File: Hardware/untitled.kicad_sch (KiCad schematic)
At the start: 7 parts, among them U8 BMP280

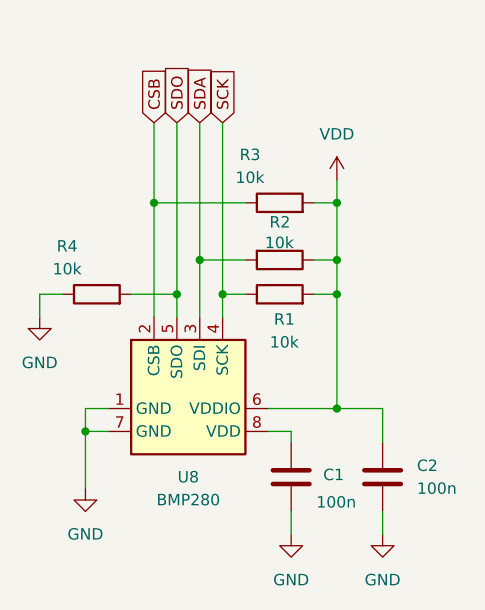
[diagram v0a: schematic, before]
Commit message: design sensores pronto
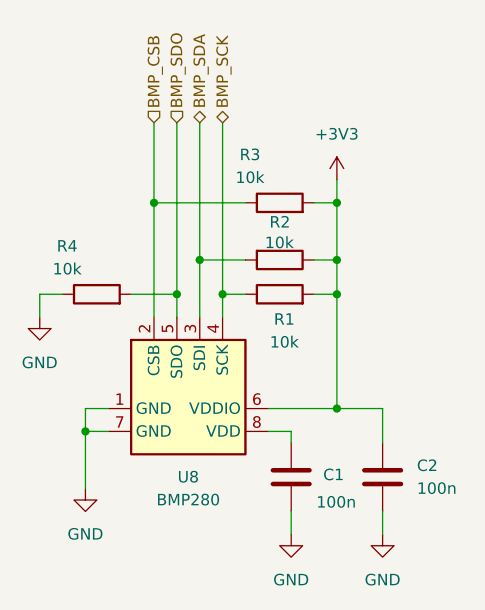
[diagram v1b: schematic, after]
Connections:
- net CSB renamed BMP_CSB
- net SCK renamed BMP_SCK
- net SDA renamed BMP_SDA
- net SDO renamed BMP_SDO
- net VDD renamed +3V3
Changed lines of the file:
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@@
 		)
 	)
-	(global_label "SDO"
+	(hierarchical_label "BMP_SDO"
 		(shape input)
 		(at 139.7 74.93 90)
-		(fields_autoplaced yes)
 		(effects
 			(font
@@
 			(justify left)
 		)
-		(property "Intersheetrefs" "${INTERSHEET_REFS}"
-			(at 139.7 68.1348 90)
-			(effects
-				(font
-					(size 1.27 1.27)
-				)
-				(justify left)
-				(hide yes)
-			)
-		)
-	)
-	(global_label "SDA"
-		(shape input)
+	)
+	(hierarchical_label "BMP_SDA"
+		(shape bidirectional)
 		(at 142.24 74.93 90)
-		(fields_autoplaced yes)
 		(effects
 			(font
@@
 			(justify left)
 		)
-		(property "Intersheetrefs" "${INTERSHEET_REFS}"
-			(at 142.24 68.3767 90)
-			(effects
-				(font
-					(size 1.27 1.27)
-				)
-				(justify left)
-				(hide yes)
-			)
-		)
-	)
-	(global_label "CSB"
+	)
+	(hierarchical_label "BMP_CSB"
 		(shape input)
 		(at 137.16 74.93 90)
-		(fields_autoplaced yes)
 		(effects
 			(font
@@
 			(justify left)
 		)
-		(property "Intersheetrefs" "${INTERSHEET_REFS}"
-			(at 137.16 68.1953 90)
-			(effects
-				(font
-					(size 1.27 1.27)
-				)
-				(justify left)
-				(hide yes)
-			)
-		)
-	)
-	(global_label "SCK"
-		(shape input)
+	)
+	(hierarchical_label "BMP_SCK"
+		(shape bidirectional)
 		(at 144.78 74.93 90)
-		(fields_autoplaced yes)
 		(effects
 			(font
@@
 			)
 			(justify left)
-		)
-		(property "Intersheetrefs" "${INTERSHEET_REFS}"
-			(at 144.78 68.1953 90)
-			(effects
-				(font
-					(size 1.27 1.27)
-				)
-				(justify left)
-				(hide yes)
-			)
 		)
 	)
@@
 	)
 	(symbol
+		(lib_id "power:+3V3")
+		(at 157.48 81.28 0)
+		(unit 1)
+		(exclude_from_sim no)
+		(in_bom yes)
+		(on_board yes)
+		(dnp no)
+		(fields_autoplaced yes)
+		(property "Reference" "#PWR015"
+			(at 157.48 85.09 0)
+			(effects
+				(font
+					(size 1.27 1.27)
+				)
+				(hide yes)
+			)
+		)
+		(property "Value" "+3V3"
+			(at 157.48 76.2 0)
+			(effects
+				(font
+					(size 1.27 1.27)
+				)
+			)
+		)
+		(property "Footprint" ""
+			(at 157.48 81.28 0)
+			(effects
+				(font
+					(size 1.27 1.27)
+				)
+				(hide yes)
+			)
+		)
+		(property "Datasheet" ""
+			(at 157.48 81.28 0)
+			(effects
+				(font
+					(size 1.27 1.27)
+				)
+				(hide yes)
+			)
+		)
+		(property "Description" "Power symbol creates a global label with name \"+3V3\""
+			(at 157.48 81.28 0)
+			(effects
+				(font
+					(size 1.27 1.27)
+				)
+				(hide yes)
+			)
+		)
+		(pin "1"
+		)
+		(instances
+			(project ""
+				(path "/0c305a6e-f9cd-49a1-b146-c2956e5469b6/0abc4084-0cd9-43a4-88f9-87e0e6566acc"
+					(reference "#PWR015")
+					(unit 1)
+				)
+			)
+		)
+	)
+	(symbol
 		(lib_id "Device:R")
 		(at 151.13 90.17 270)
@@
 					(unit 1)
 				)
-			)
-		)
-	)
-	(symbol
-		(lib_id "power:VDD")
-		(at 157.48 81.28 0)
-		(unit 1)
-		(exclude_from_sim no)
-		(in_bom yes)
-		(on_board yes)
-		(dnp no)
-		(fields_autoplaced yes)
-		(property "Reference" "#PWR016"
-			(at 157.48 85.09 0)
-			(effects
-				(font
-					(size 1.27 1.27)
-				)
-				(hide yes)
-			)
-		)
-		(property "Value" "VDD"
-			(at 157.48 76.2 0)
-			(effects
-				(font
-					(size 1.27 1.27)
-				)
-			)
-		)
-		(property "Footprint" ""
-			(at 157.48 81.28 0)
-			(effects
-				(font
-					(size 1.27 1.27)
-				)
-				(hide yes)
-			)
-		)
-		(property "Datasheet" ""
-			(at 157.48 81.28 0)
-			(effects
-				(font
-					(size 1.27 1.27)
-				)
-				(hide yes)
-			)
-		)
-		(property "Description" "Power symbol creates a global label with name \"VDD\""
-			(at 157.48 81.28 0)
-			(effects
-				(font
-					(size 1.27 1.27)
-				)
-				(hide yes)
-			)
-		)
-		(pin "1"
-		)
-		(instances
-			(project ""
-				(path "/0c305a6e-f9cd-49a1-b146-c2956e5469b6/0abc4084-0cd9-43a4-88f9-87e0e6566acc"
-					(reference "#PWR016")
-					(unit 1)
-				)
